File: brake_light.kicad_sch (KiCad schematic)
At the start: 2 parts, among them U1 US2881LUA-AAA-000-BU, U2 US2881LUA-AAA-000-BU

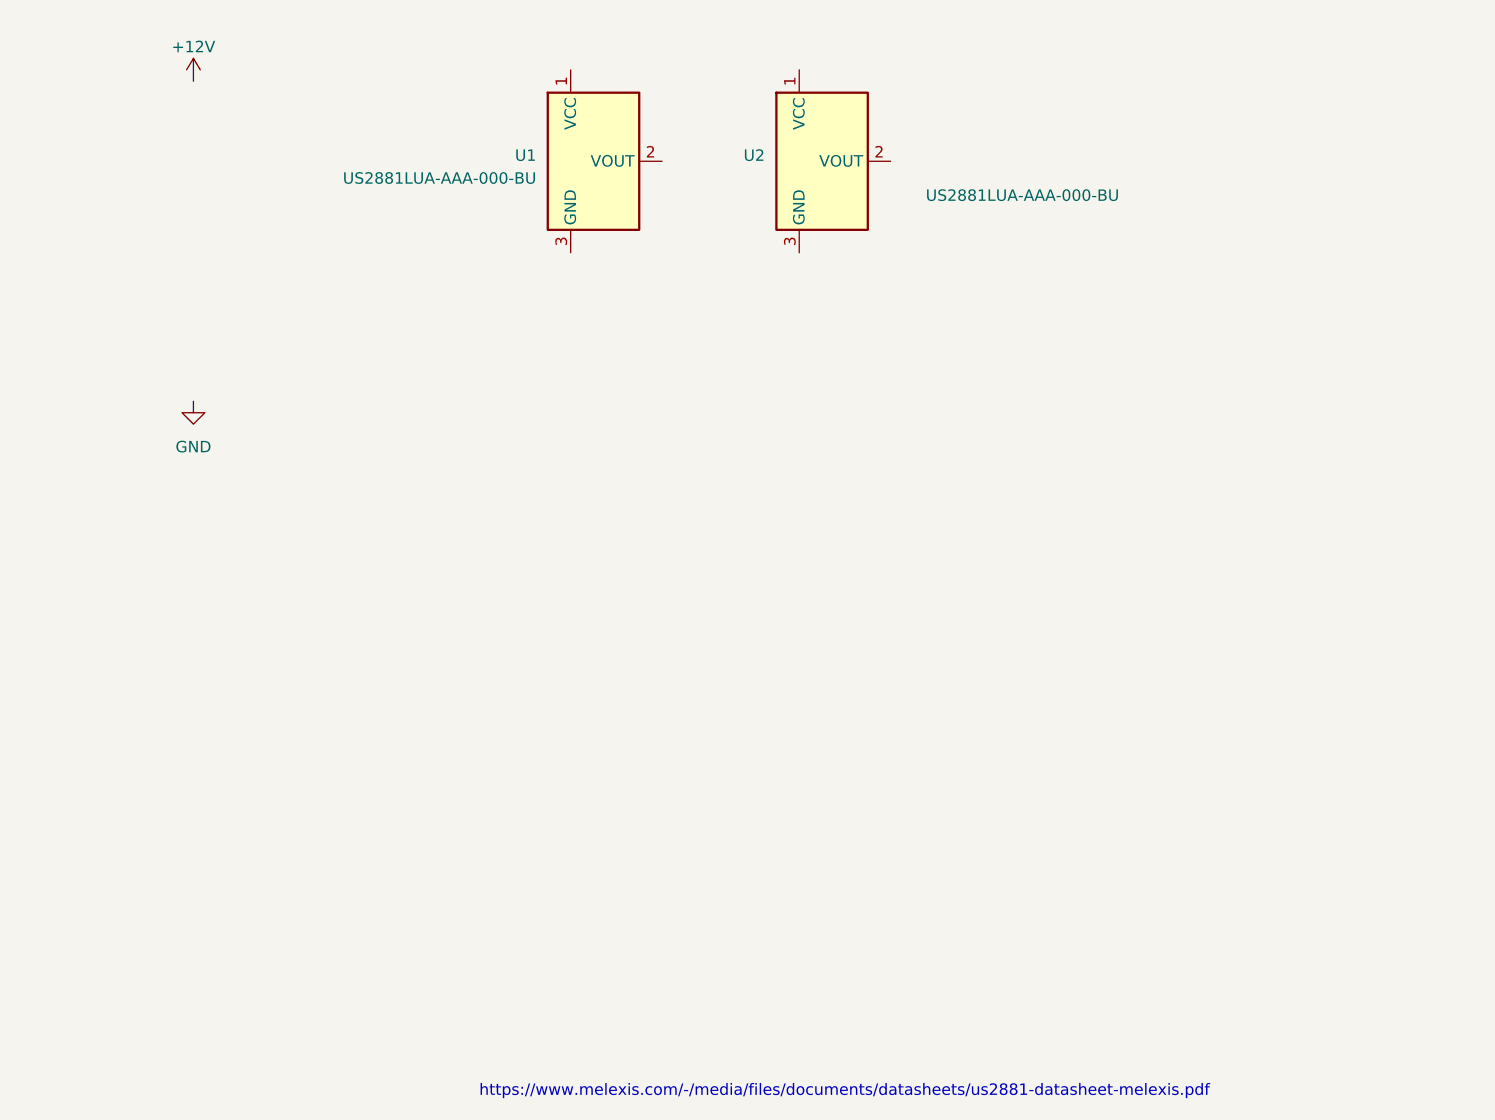
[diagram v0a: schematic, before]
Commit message: first commit
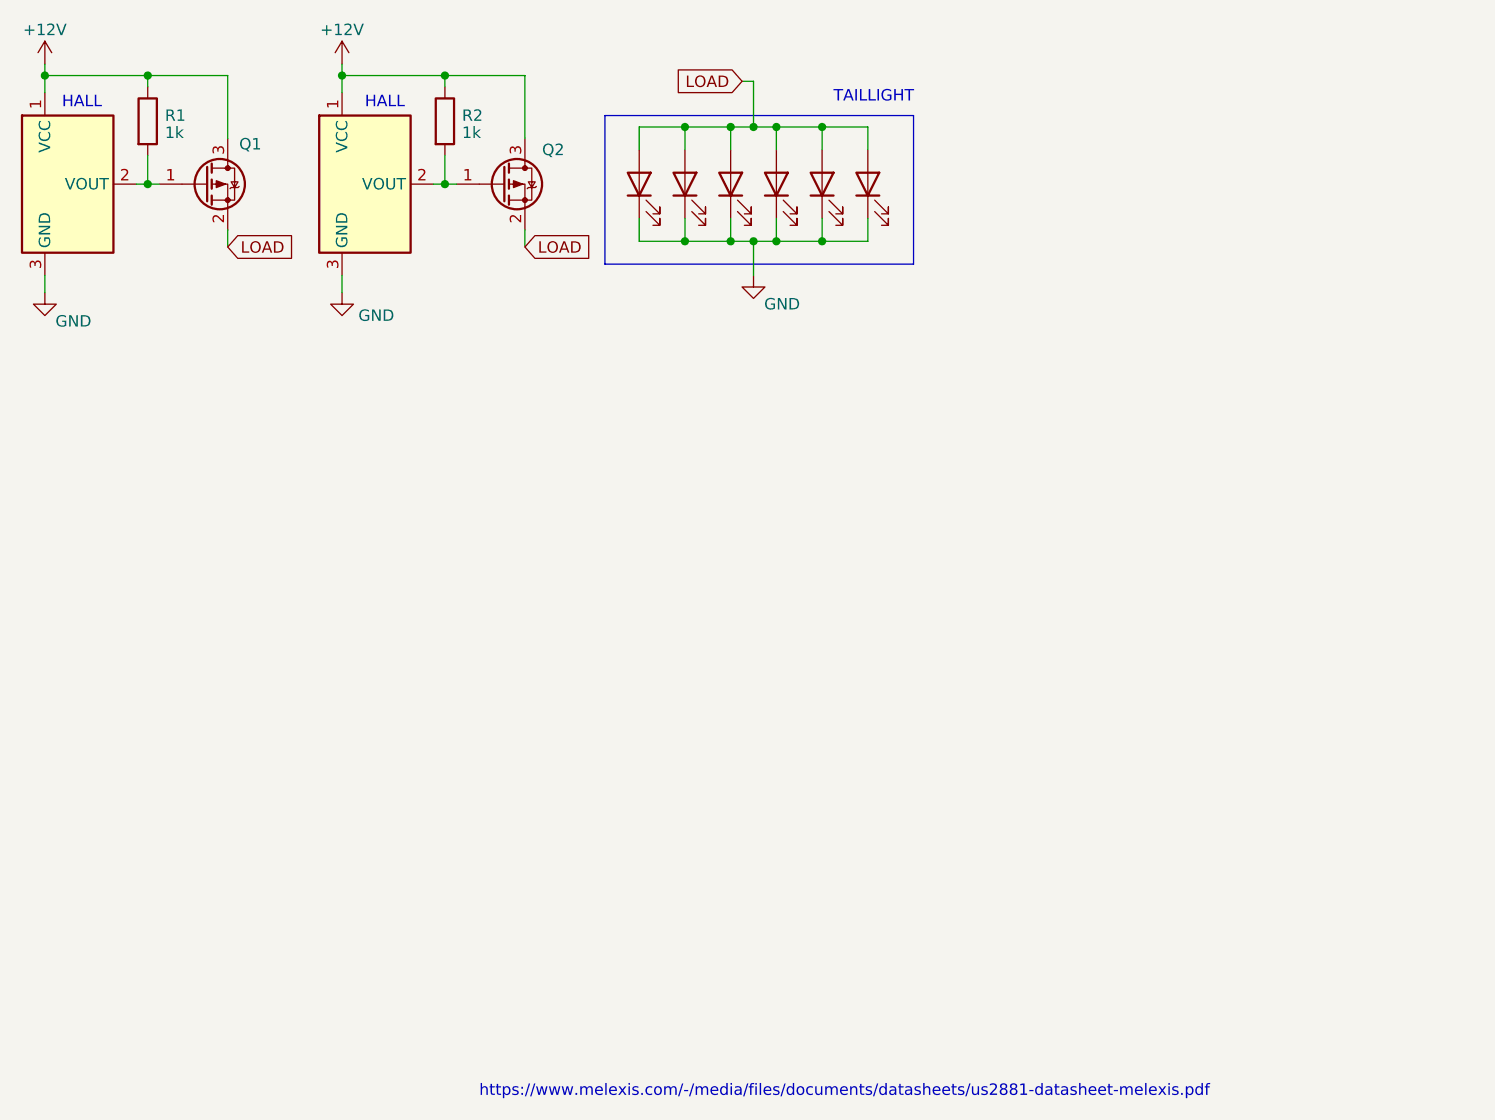
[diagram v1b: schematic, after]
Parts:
- added D1, D2, D3, D4, D5, D6: LED, symbol Device:LED
- added Q1, Q2: AO3401A, Package_TO_SOT_SMD:SOT-23, symbol Transistor_FET:AO3401A
- added R1, R2: 1k, symbol Device:R
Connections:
- net +12V: now also U1.1 (VCC), U2.1 (VCC), Q1.3 (D), Q2.3 (D), R1.1, R2.1
- net GND: now also U1.3 (GND), U2.3 (GND), D1.1 (K), D2.1 (K), D3.1 (K), D4.1 (K), D5.1 (K), D6.1 (K)
- net at U2.2 (VOUT): now also Q2.1 (G), R2.2
- net at U1.2 (VOUT): now also Q1.1 (G), R1.2
- new net LOAD: D1.2 (A), D2.2 (A), D3.2 (A), D4.2 (A), D5.2 (A), D6.2 (A), Q1.2 (S), Q2.2 (S)
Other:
- note added: "HALL"
- note added: "TAILLIGHT"
